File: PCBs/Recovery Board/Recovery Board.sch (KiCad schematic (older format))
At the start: 16 parts, among them J1 Conn_01x02, J2 Conn_01x02, J3 Conn_01x02, J4 Conn_01x02, J5 Conn_01x02, U1 R-78E3.3-0.5, X1 XBee-S2C

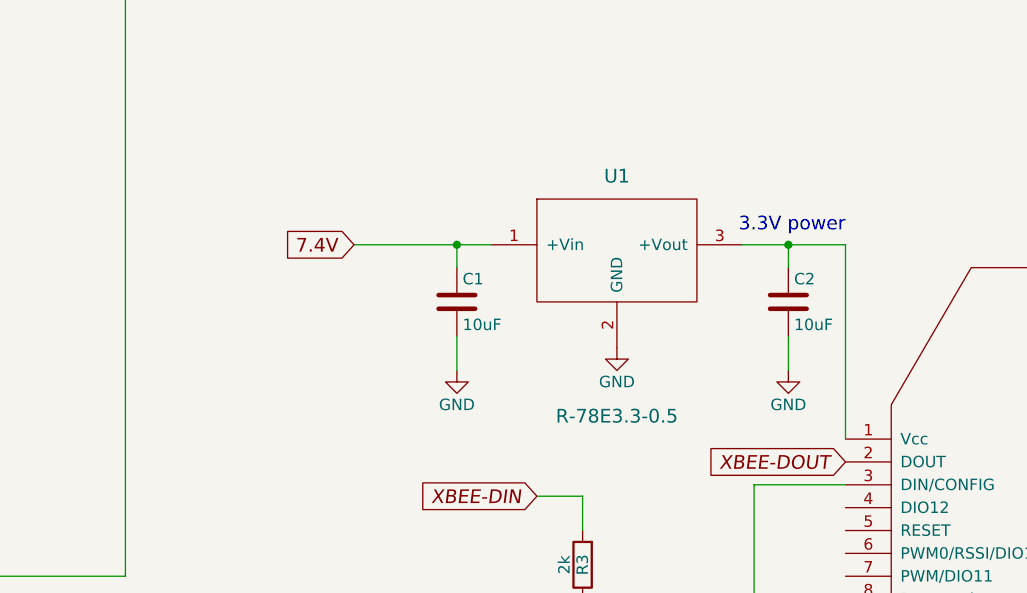
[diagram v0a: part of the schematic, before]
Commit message: stashing changes
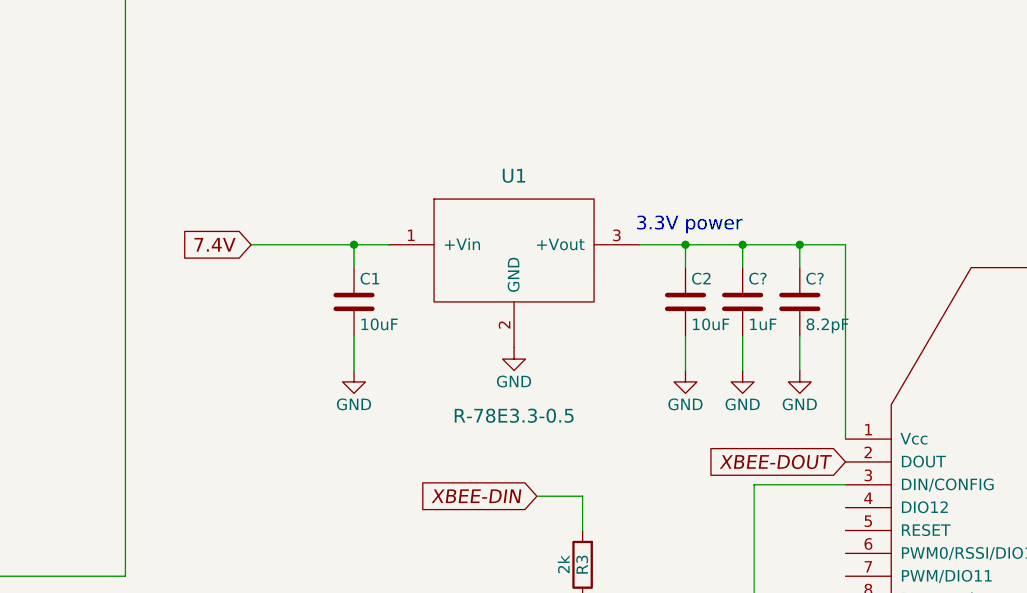
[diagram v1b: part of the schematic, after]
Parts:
- added C?: 1uF, Capacitors_SMD:C_0805_HandSoldering, symbol C
- added C?: 8.2pF, Capacitors_SMD:C_0805_HandSoldering, symbol C
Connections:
- net GND: now also C?.2, C?.2
- net at C2.1, U1.3 (+Vout), X1.1 (Vcc): now also C?.1, C?.1
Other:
- moved on the sheet: C1, C2, U1
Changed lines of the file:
@@
 SCL
 Wire Wire Line
-	7300 4200 7750 4200
+	6850 4200 7750 4200
 $Comp
 L CPC1002N S1
@@
 Wire Wire Line
 	6600 6450 6600 6600
-Text GLabel 5600 4200 0    60   Input ~ 0
+Text GLabel 5150 4200 0    60   Input ~ 0
 7.4V
 Wire Wire Line
@@
 Connection ~ 6900 2400
 Wire Wire Line
-	7500 4750 7500 4750
-Wire Wire Line
-	7500 4750 7500 4600
-Wire Wire Line
-	7500 4300 7500 4200
-Connection ~ 7500 4200
+	7050 4750 7050 4750
+Wire Wire Line
+	7050 4750 7050 4600
+Wire Wire Line
+	7050 4300 7050 4200
+Connection ~ 7050 4200
 Text Notes 7200 5850 2    60   ~ 0
 3.3V data
-Text Notes 7750 4150 2    60   ~ 0
+Text Notes 7300 4150 2    60   ~ 0
 3.3V power
-Connection ~ 6050 4200
+Connection ~ 5600 4200
 $Comp
 L Conn_01x02 J5
@@
 L GND #PWR02
 U 1 1 5A9AC98C
-P 6050 4750
-F 0 "#PWR02" H 6050 4500 50  0001 C CNN
-F 1 "GND" H 6050 4600 50  0000 C CNN
-F 2 "" H 6050 4750 50  0001 C CNN
-F 3 "" H 6050 4750 50  0001 C CNN
-	1    6050 4750
+P 5600 4750
+F 0 "#PWR02" H 5600 4500 50  0001 C CNN
+F 1 "GND" H 5600 4600 50  0000 C CNN
+F 2 "" H 5600 4750 50  0001 C CNN
+F 3 "" H 5600 4750 50  0001 C CNN
+	1    5600 4750
 	1    0    0    -1
 $EndComp
@@
 L GND #PWR03
 U 1 1 5A9ACBA8
-P 6750 4650
-F 0 "#PWR03" H 6750 4400 50  0001 C CNN
-F 1 "GND" H 6750 4500 50  0000 C CNN
-F 2 "" H 6750 4650 50  0001 C CNN
-F 3 "" H 6750 4650 50  0001 C CNN
-	1    6750 4650
+P 6300 4650
+F 0 "#PWR03" H 6300 4400 50  0001 C CNN
+F 1 "GND" H 6300 4500 50  0000 C CNN
+F 2 "" H 6300 4650 50  0001 C CNN
+F 3 "" H 6300 4650 50  0001 C CNN
+	1    6300 4650
 	1    0    0    -1
 $EndComp
@@
 L GND #PWR05
 U 1 1 5A9AD339
-P 7500 4750
-F 0 "#PWR05" H 7500 4500 50  0001 C CNN
-F 1 "GND" H 7500 4600 50  0000 C CNN
-F 2 "" H 7500 4750 50  0001 C CNN
-F 3 "" H 7500 4750 50  0001 C CNN
-	1    7500 4750
+P 7050 4750
+F 0 "#PWR05" H 7050 4500 50  0001 C CNN
+F 1 "GND" H 7050 4600 50  0000 C CNN
+F 2 "" H 7050 4750 50  0001 C CNN
+F 3 "" H 7050 4750 50  0001 C CNN
+	1    7050 4750
 	1    0    0    -1
 $EndComp
@@
 L C C1
 U 1 1 5A9AEA7D
-P 6050 4450
-F 0 "C1" H 6075 4550 50  0000 L CNN
-F 1 "10uF" H 6075 4350 50  0000 L CNN
-F 2 "Capacitors_SMD:C_0805_HandSoldering" H 6088 4300 50  0001 C CNN
-F 3 "" H 6050 4450 50  0001 C CNN
-	1    6050 4450
+P 5600 4450
+F 0 "C1" H 5625 4550 50  0000 L CNN
+F 1 "10uF" H 5625 4350 50  0000 L CNN
+F 2 "Capacitors_SMD:C_0805_HandSoldering" H 5638 4300 50  0001 C CNN
+F 3 "" H 5600 4450 50  0001 C CNN
+	1    5600 4450
 	1    0    0    -1
 $EndComp
@@
 L C C2
 U 1 1 5A9AEB07
-P 7500 4450
-F 0 "C2" H 7525 4550 50  0000 L CNN
-F 1 "10uF" H 7525 4350 50  0000 L CNN
-F 2 "Capacitors_SMD:C_0805_HandSoldering" H 7538 4300 50  0001 C CNN
-F 3 "" H 7500 4450 50  0001 C CNN
-	1    7500 4450
+P 7050 4450
+F 0 "C2" H 7075 4550 50  0000 L CNN
+F 1 "10uF" H 7075 4350 50  0000 L CNN
+F 2 "Capacitors_SMD:C_0805_HandSoldering" H 7088 4300 50  0001 C CNN
+F 3 "" H 7050 4450 50  0001 C CNN
+	1    7050 4450
 	1    0    0    -1
 $EndComp
@@
 L R-78E3.3-0.5 U1
 U 1 1 5A9B412D
-P 6750 4350
-F 0 "U1" H 6750 4800 60  0000 C CNN
-F 1 "R-78E3.3-0.5" H 6750 3750 60  0000 C CNN
-F 2 "sip:SIP3" H 6750 4350 60  0001 C CNN
-F 3 "" H 6750 4350 60  0001 C CNN
-	1    6750 4350
-	1    0    0    -1
-$EndComp
-Wire Wire Line
-	5600 4200 6200 4200
-Wire Wire Line
-	6050 4300 6050 4200
-Wire Wire Line
-	6050 4600 6050 4750
+P 6300 4350
+F 0 "U1" H 6300 4800 60  0000 C CNN
+F 1 "R-78E3.3-0.5" H 6300 3750 60  0000 C CNN
+F 2 "sip:SIP3" H 6300 4350 60  0001 C CNN
+F 3 "" H 6300 4350 60  0001 C CNN
+	1    6300 4350
+	1    0    0    -1
+$EndComp
+Wire Wire Line
+	5150 4200 5750 4200
+Wire Wire Line
+	5600 4300 5600 4200
+Wire Wire Line
+	5600 4600 5600 4750
+Wire Wire Line
+	7300 4750 7300 4750
+Wire Wire Line
+	7300 4750 7300 4600
+Wire Wire Line
+	7300 4200 7300 4300
+$Comp
+L GND #PWR?
+U 1 1 5ABA400A
+P 7300 4750
+F 0 "#PWR?" H 7300 4500 50  0001 C CNN
+F 1 "GND" H 7300 4600 50  0000 C CNN
+F 2 "" H 7300 4750 50  0001 C CNN
+F 3 "" H 7300 4750 50  0001 C CNN
+	1    7300 4750
+	1    0    0    -1
+$EndComp
+$Comp
+L C C?
+U 1 1 5ABA4010
+P 7300 4450
+F 0 "C?" H 7325 4550 50  0000 L CNN
+F 1 "1uF" H 7325 4350 50  0000 L CNN
+F 2 "Capacitors_SMD:C_0805_HandSoldering" H 7338 4300 50  0001 C CNN
+F 3 "" H 7300 4450 50  0001 C CNN
+	1    7300 4450
+	1    0    0    -1
+$EndComp
+Wire Wire Line
+	7550 4750 7550 4750
+Wire Wire Line
+	7550 4750 7550 4600
+Wire Wire Line
+	7550 4200 7550 4300
+$Comp
+L GND #PWR?
+U 1 1 5ABA4092
+P 7550 4750
+F 0 "#PWR?" H 7550 4500 50  0001 C CNN
+F 1 "GND" H 7550 4600 50  0000 C CNN
+F 2 "" H 7550 4750 50  0001 C CNN
+F 3 "" H 7550 4750 50  0001 C CNN
+	1    7550 4750
+	1    0    0    -1
+$EndComp
+$Comp
+L C C?
+U 1 1 5ABA4098
+P 7550 4450
+F 0 "C?" H 7575 4550 50  0000 L CNN
+F 1 "8.2pF" H 7575 4350 50  0000 L CNN
+F 2 "Capacitors_SMD:C_0805_HandSoldering" H 7588 4300 50  0001 C CNN
+F 3 "" H 7550 4450 50  0001 C CNN
+	1    7550 4450
+	1    0    0    -1
+$EndComp
+Connection ~ 7300 4200
+Connection ~ 7550 4200
 $EndSCHEMATC
